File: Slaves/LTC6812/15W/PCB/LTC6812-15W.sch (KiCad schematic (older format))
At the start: 55 parts, among them J1 Conn_01x01, J10 Slave, J11 Master, J2 Conn_01x01, J3 Conn_01x01, J4 Conn_01x01, J5 Cells, J6 Conn_01x10, Q1 DZTT5551, U1 LTC6812

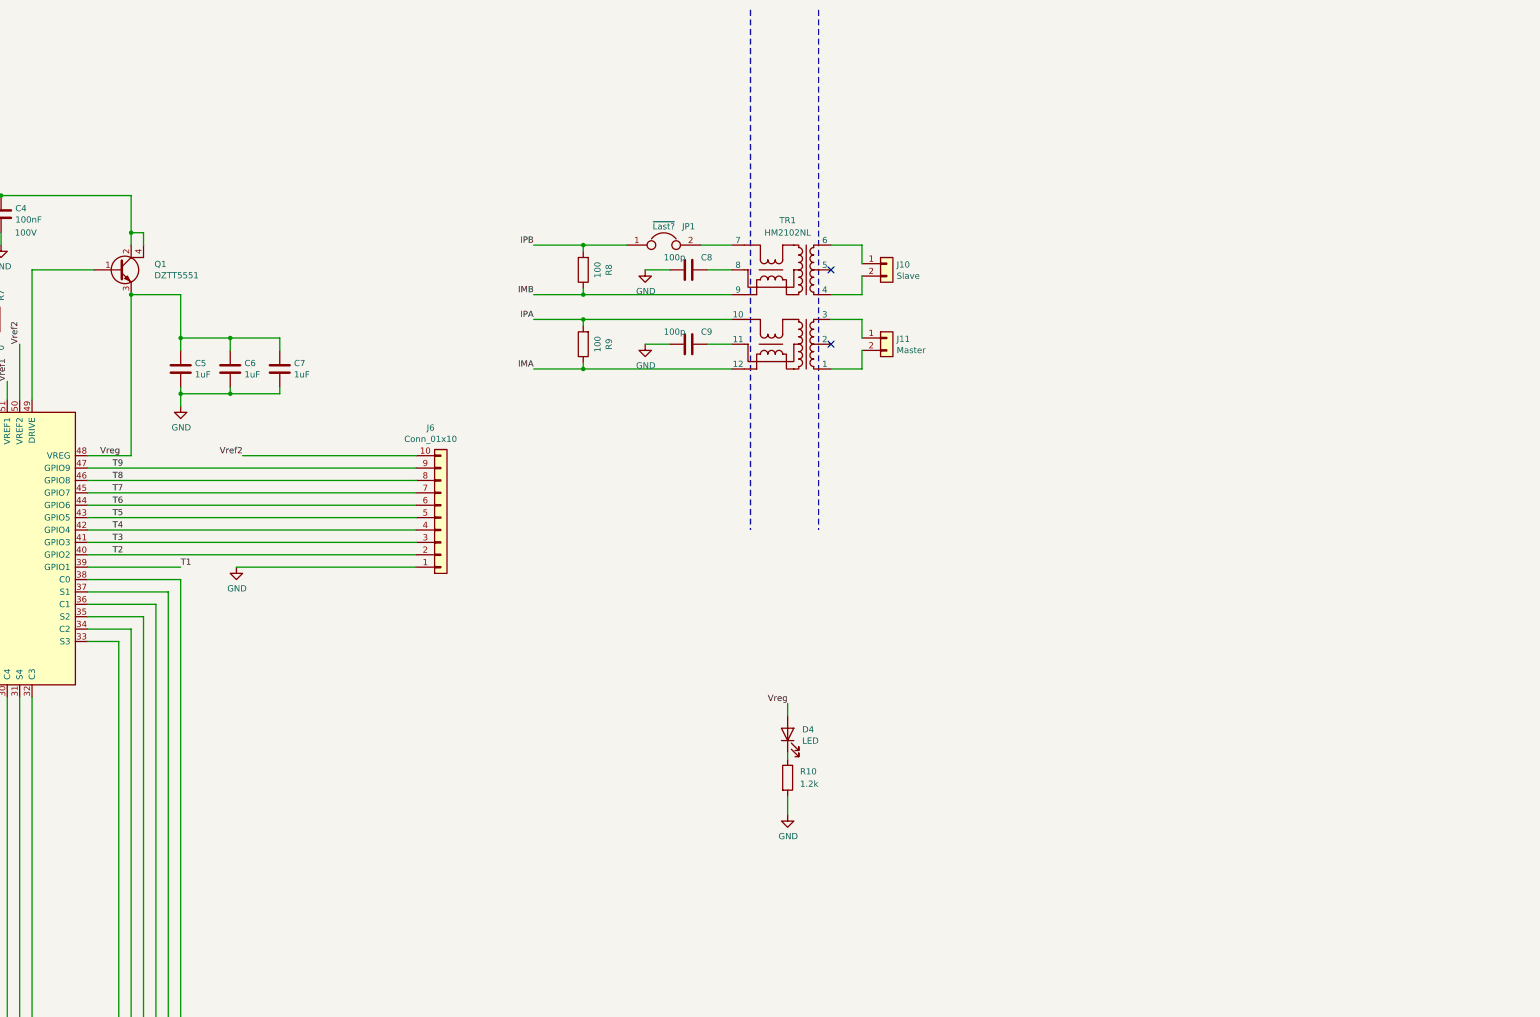
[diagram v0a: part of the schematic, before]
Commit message: Readme changes
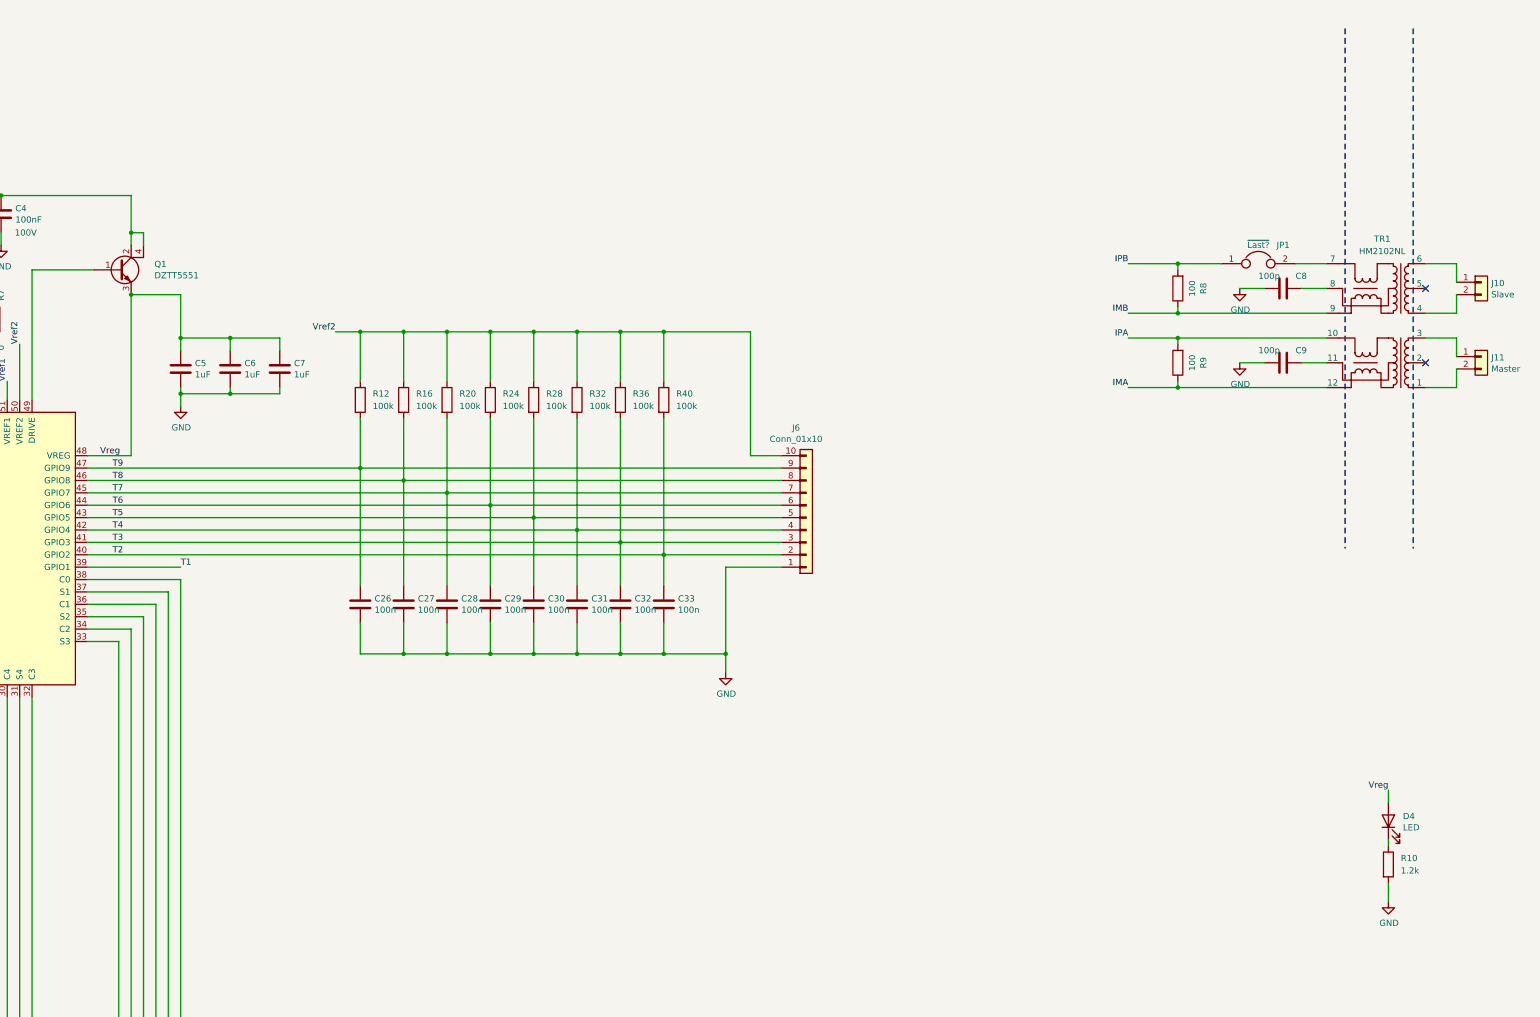
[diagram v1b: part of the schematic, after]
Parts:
- added C26, C27, C28, C29, C30, C31, C32, C33: 100n, Capacitors_SMD:C_0603_HandSoldering, symbol Device:C
- added R12, R16, R20, R24, R28, R32, R36, R40: 100k, Resistors_SMD:R_0603_HandSoldering, symbol Device:R
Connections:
- net GND: now also C26.2, C27.2, C28.2, C29.2, C30.2, C31.2, C32.2, C33.2
- net T2: now also C33.1, R40.2
- net T3: now also C32.1, R36.2
- net T4: now also C31.1, R32.2
- net T5: now also C30.1, R28.2
- net T6: now also C29.1, R24.2
- net T7: now also C28.1, R20.2
- net T8: now also C27.1, R16.2
- net T9: now also C26.1, R12.2
- net Vref2: now also R12.1, R16.1, R20.1, R24.1, R28.1, R32.1, R36.1, R40.1
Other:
- moved on the sheet: C8, C9, D4, J10, J11, J6, JP1, R10, R8, R9, TR1
